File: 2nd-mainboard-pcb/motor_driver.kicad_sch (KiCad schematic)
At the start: 4 parts, among them J15 Stepper Motor, J2 Servo Motor, U4 MPU-6050

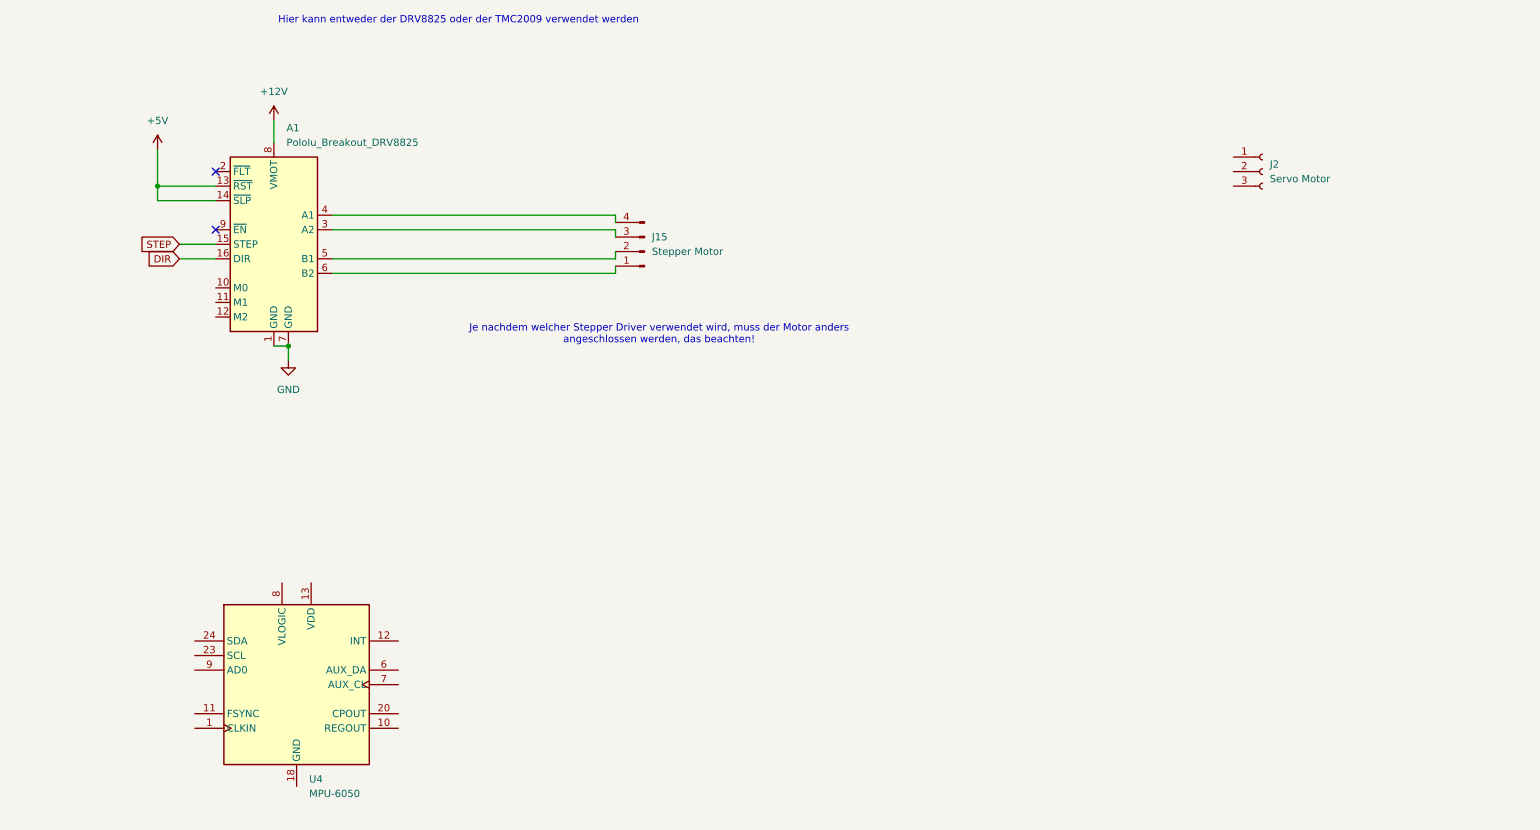
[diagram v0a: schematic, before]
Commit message: finished stacked design, annotaded
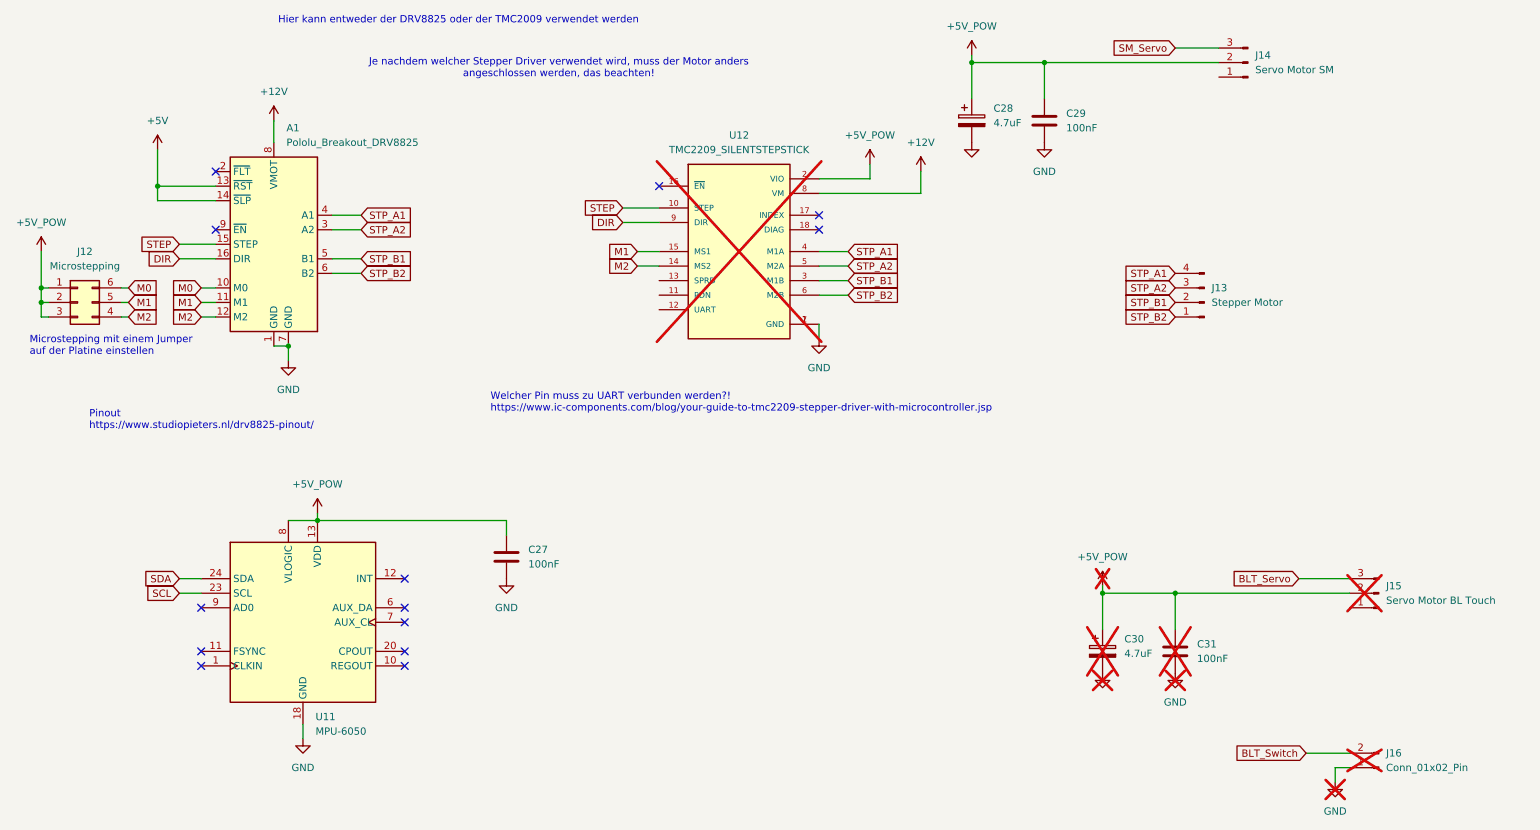
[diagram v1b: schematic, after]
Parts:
- removed J2: Servo Motor, symbol Connector:Conn_01x03_Socket
- added C27, C29, C31: 100nF, symbol Device:C
- added C28, C30: 4.7uF, symbol Device:C_Polarized
- added J12: Microstepping, symbol Connector_Generic:Conn_02x03_Counter_Clockwise
- added J14: Servo Motor SM, Imported_Component_Footprints:JST_XH_S3B-XH-A_1x03_P2.50mm_Horizontal, symbol Connector:Conn_01x03_Pin
- added J15: Servo Motor BL Touch, symbol Connector:Conn_01x03_Pin
- added J16: Conn_01x02_Pin, symbol Connector:Conn_01x02_Pin
- added U12: TMC2209_SILENTSTEPSTICK, Imported_Component_Footprints:MODULE_TMC2209_SILENTSTEPSTICK, symbol Imported_Component_Symbols:TMC2209_SILENTSTEPSTICK
- J13: renamed from J15; footprint (none) -> Imported_Component_Footprints:JST_S4B-XH-A-1
- renumbered U4 to U11
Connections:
- net +12V: now also U12.8 (VM)
- net DIR: now also U12.9 (DIR)
- net GND: now also U11.18 (GND), C27.2, C28.2, C29.2, C30.2, C31.2, J16.1 (Pin_1), U12.1 (GND), U12.7 (GND)
- net STEP: now also U12.10 (STEP)
- net M0: now reaches A1.10 (M0)
- net M0: now also J12.6 (Pin_6)
- net M1: now reaches A1.11 (M1)
- net M1: now also J12.5 (Pin_5), U12.15 (MS1)
- net M2: now reaches A1.12 (M2)
- net M2: now also J12.4 (Pin_4), U12.14 (MS2)
- net STP_A2: now reaches A1.3 (A2), J13.3 (Pin_3)
- net STP_A2: now also U12.5 (M2A)
- net STP_A1: now reaches A1.4 (A1), J13.4 (Pin_4)
- net STP_A1: now also U12.4 (M1A)
- net STP_B1: now reaches A1.5 (B1), J13.2 (Pin_2)
- net STP_B1: now also U12.3 (M1B)
- net STP_B2: now reaches A1.6 (B2), J13.1 (Pin_1)
- net STP_B2: now also U12.6 (M2B)
- net +5V_POW: now reaches U11.13 (VDD)
- net +5V_POW: now also U11.8 (VLOGIC), C27.1, C28.1, C29.1, C30.1, C31.1, J12.1 (Pin_1), J12.2 (Pin_2), J12.3 (Pin_3), J14.2 (Pin_2), J15.2 (Pin_2), U12.2 (VIO)
- net SCL: now reaches U11.23 (SCL)
- net SDA: now reaches U11.24 (SDA)
- new net BLT_Servo: J15.3 (Pin_3)
- new net BLT_Switch: J16.2 (Pin_2)
- new net SM_Servo: J14.3 (Pin_3)
- no-connect marks 2 -> 13
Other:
- note added: "Microstepping mit einem Jumper auf der Platine einstellen"
- note added: "Pinout https://www.studiopieters.nl/drv8825-pinout/"
- note added: "Welcher Pin muss zu UART verbunden werden?! https://www.ic-components.com/blog/your-guide-to-tmc2209-stepper-driver-with-microcontroller.jsp"
- moved on the sheet: J13, U11
